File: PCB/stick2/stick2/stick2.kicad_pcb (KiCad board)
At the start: 2 copper layers, 80 x 65.5 mm, 13 parts, among them J1 Conn_01x08_Pin, U1 MLX90395xLW

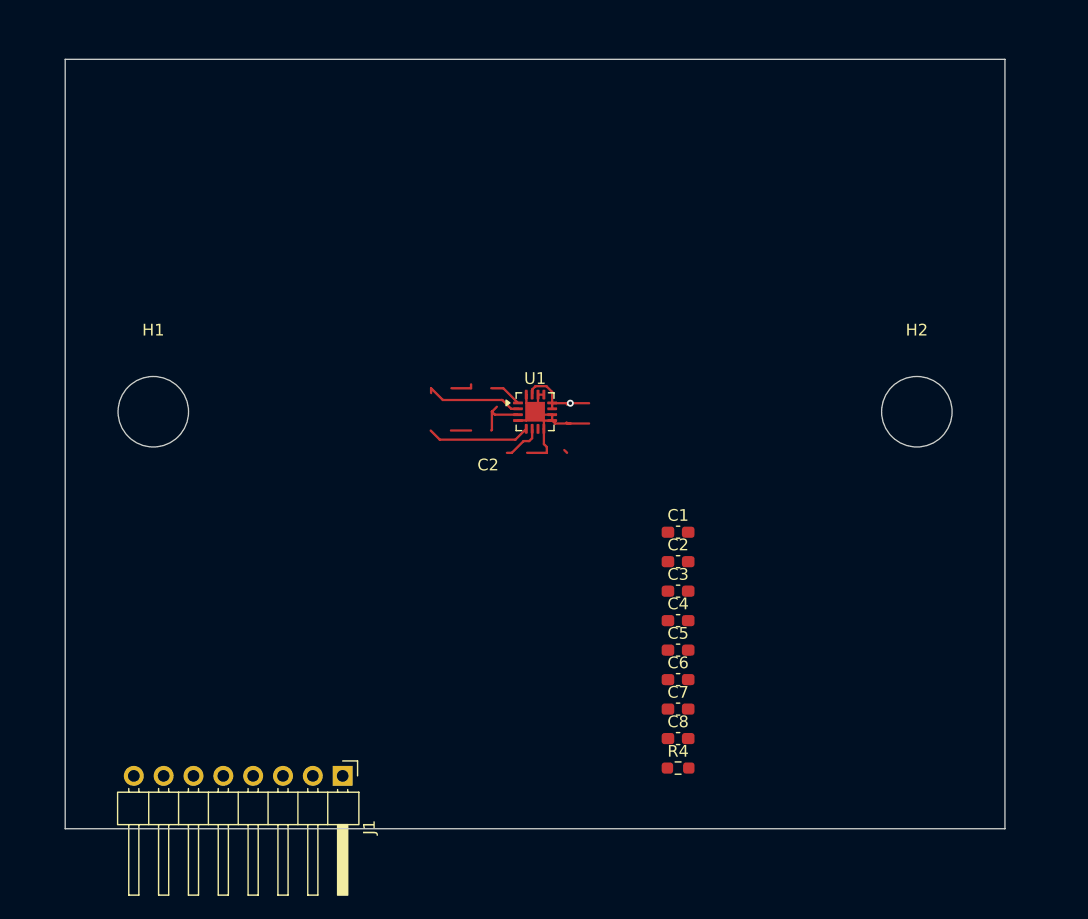
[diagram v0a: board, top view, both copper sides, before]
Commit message: boards
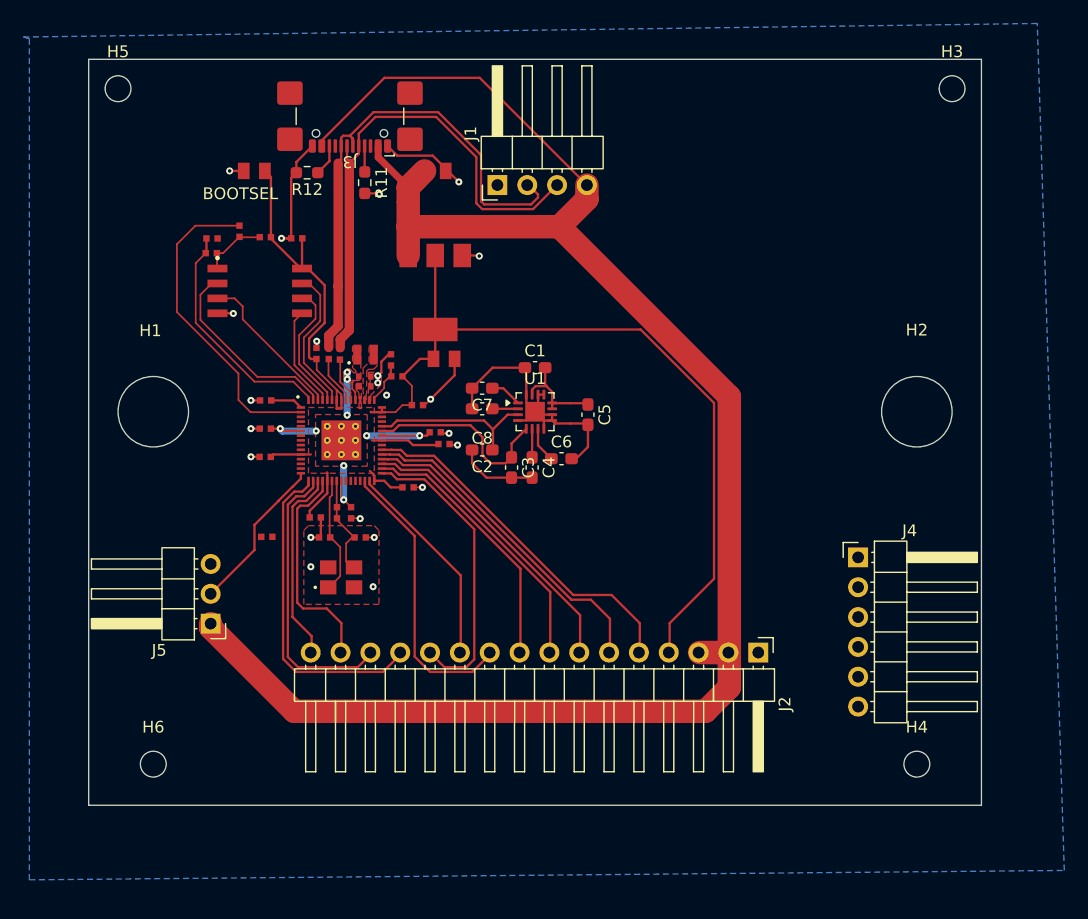
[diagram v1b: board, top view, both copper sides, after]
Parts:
- removed R4: 100, Resistor_SMD:R_0603_1608Metric_Pad0.98x0.95mm_HandSolder
- added C10: 100n, RPI_COMPILED:generic_capc1005x50, F.Cu at (117.1, 79.0)
- added C11: 10u, RPI_COMPILED:generic_capc2012x125, F.Cu at (132.2, 75.5)
- added C12: 15p, RPI_COMPILED:generic_capc1005x50, F.Cu at (122.1, 90.7)
- added C13: 15p, RPI_COMPILED:generic_capc1005x50, F.Cu at (125.1, 90.7)
- added C14: 100n, RPI_COMPILED:generic_capc1005x50, F.Cu at (124.3, 88.6)
- added C15: 100n, RPI_COMPILED:generic_capc1005x50, F.Cu at (131.5, 81.8)
- added C16: 100n, RPI_COMPILED:generic_capc1005x50, F.Cu at (117.0, 81.4)
- added C17: 4.7u, RPI_COMPILED:generic_capc1005x50_wide, F.Cu at (125.5, 77.0)
- added C18: 4.7u, RPI_COMPILED:generic_capc1005x50_wide, F.Cu at (125.5, 77.8)
- added C19: 4.7u, RPI_COMPILED:generic_capc1005x50, F.Cu at (127.7, 75.6)
- added C20: 100n, RPI_COMPILED:generic_capc1005x50, F.Cu at (121.4, 75.0)
- added C21: 100n, RPI_COMPILED:generic_capc1005x50, F.Cu at (130.0, 79.4)
- added C22: 10u, RPI_COMPILED:generic_capc2012x125, F.Cu at (116.1, 59.5)
- added C23: 100n, RPI_COMPILED:generic_capc1005x50, F.Cu at (129.2, 86.4)
- added C24: 100n, RPI_COMPILED:generic_capc1005x50, F.Cu at (121.3, 89.0)
- added C25: 100n, RPI_COMPILED:generic_capc1005x50, F.Cu at (132.2, 82.8)
- added C26: 100n, RPI_COMPILED:generic_capc1005x50, F.Cu at (119.7, 65.2)
- added C27: 100n, RPI_COMPILED:generic_capc1005x50, F.Cu at (117.0, 83.8)
- added C9: 10u, RPI_COMPILED:generic_capc2012x125, F.Cu at (131.5, 59.5)
- added H3: MountingHole, MountingHole:MountingHole_2.2mm_M2, F.Cu at (175.5, 52.5)
- added H4: MountingHole, MountingHole:MountingHole_2.2mm_M2, F.Cu at (172.5, 110.0)
- added H5: MountingHole, MountingHole:MountingHole_2.2mm_M2, F.Cu at (104.5, 52.5)
- added H6: MountingHole, MountingHole:MountingHole_2.2mm_M2, F.Cu at (107.5, 110.0)
- added J2: Conn_01x16, Connector_PinHeader_2.54mm:PinHeader_1x16_P2.54mm_Horizontal, F.Cu at (159.0, 100.5)
- added J3: USB_C_Receptacle_USB2.0_16P, Connector_USB:USB_C_Receptacle_GCT_USB4110, F.Cu at (124.2, 53.7)
- added J4: Conn_01x06_Pin, Connector_PinHeader_2.54mm:PinHeader_1x06_P2.54mm_Horizontal, F.Cu at (167.5, 92.4)
- added J5: Conn_01x03_Pin, Connector_PinHeader_2.54mm:PinHeader_1x03_P2.54mm_Horizontal, F.Cu at (112.4, 98.0)
- added L1: 3.3u, RPI_COMPILED:abracon_aota-b201610s3r3-101-t, F.Cu at (125.6, 75.1)
- added R1: 10k, RPI_COMPILED:generic_resc1005x35, F.Cu at (117.0, 65.1)
- added R10: 0, RPI_COMPILED:generic_resc1005x35, F.Cu at (112.4, 66.5)
- added R11: 5.1k, Resistor_SMD:R_0603_1608Metric_Pad0.98x0.95mm_HandSolder, F.Cu at (125.5, 60.5)
- added R12: 5.1k, Resistor_SMD:R_0603_1608Metric_Pad0.98x0.95mm_HandSolder, F.Cu at (120.6, 59.7)
- added R2: 1k, RPI_COMPILED:generic_resc1005x35, F.Cu at (123.1, 88.6)
- added R3: 33, RPI_COMPILED:generic_resc1005x35, F.Cu at (128.2, 77.0)
- added R5: 1k, RPI_COMPILED:generic_resc1005x35, F.Cu at (117.2, 90.7)
- added R6: 1k, RPI_COMPILED:generic_resc1005x35, F.Cu at (112.5, 65.2)
- added R7: 27, RPI_COMPILED:generic_resc1005x35, F.Cu at (122.4, 75.0)
- added R8: 27, RPI_COMPILED:generic_resc1005x35, F.Cu at (123.4, 75.1)
- added R9: 0, RPI_COMPILED:generic_resc1005x35, F.Cu at (114.8, 64.6)
- added U2: NCP1117ST33T3G, RPI_COMPILED:onsemi_ncp1117st33t3g, F.Cu at (131.5, 69.8)
- added U3: W25Q128JVSIQ, RPI_COMPILED:generic_soic127p790x195-8, F.Cu at (116.6, 69.7)
- added U4: RP2350A, RPI_COMPILED:rpi_rp2350a_vias, F.Cu at (123.5, 82.4)
- added X1: 12MHz, RPI_COMPILED:generic_xtalcc320x250x80-4, F.Cu at (123.5, 94.1)
- J1: value Conn_01x08_Pin -> Conn_01x04_Pin; footprint Connector_PinHeader_2.54mm:PinHeader_1x08_P2.54mm_Horizontal -> Connector_PinHeader_2.54mm:PinHeader_1x04_P2.54mm_Horizontal
- moved J1 52.0 mm to (136.8, 60.7), turned to 90 degrees
- moved C8 32.7 mm to (135.5, 79.8), turned to 180 degrees
- moved C7 32.0 mm to (135.5, 78.0), turned to 180 degrees
- moved C5 21.5 mm to (144.5, 80.2), turned to -90 degrees
- moved C6 21.3 mm to (142.2, 84.0)
- moved C2 19.2 mm to (135.5, 83.2), turned to 180 degrees
- moved C1 18.6 mm to (140.0, 76.2)
- moved C4 18.0 mm to (139.8, 84.8), turned to -90 degrees
- moved C3 17.7 mm to (138.0, 84.8), turned to -90 degrees
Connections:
- net /CS renamed Net-(U1-~{CS})
- net /MISO renamed Net-(U1-MISO)
- net /MOSI renamed /GPIO26_ADC0
- net Net-(U1-SCLK) renamed /GPIO27_ADC1
- J1 pad 1: unconnected-(J1-Pin_1-Pad1) -> GND
- J1 pad 2: unconnected-(J1-Pin_2-Pad2) -> /USB_D+
- J1 pad 3: unconnected-(J1-Pin_3-Pad3) -> /USB_D-
- J1 pad 4: unconnected-(J1-Pin_4-Pad4) -> VBUS
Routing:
- net VBUS: track 0.00 -> 159.0 mm
- net +3V3: track 0.00 -> 117.4 mm
- net /USB_D+: track 0.00 -> 44.7 mm
- net /USB_D-: track 0.00 -> 44.3 mm
- net GND: track 0.00 -> 38.4 mm, vias 0 -> 22
- net /GPIO24: track 0.00 -> 30.7 mm
- net /GPIO23: track 0.00 -> 28.2 mm
- net /GPIO12: track 0.00 -> 27.6 mm
- net /GPIO0: track 0.00 -> 27.1 mm
- net /GPIO22: track 0.00 -> 25.7 mm
- net /GPIO19: track 0.00 -> 25.3 mm
- net +1V1: track 0.00 -> 25.3 mm, vias 0 -> 9
- net /GPIO17: track 0.00 -> 24.4 mm
- net /GPIO13: track 0.00 -> 24.2 mm
- net /GPIO21: track 0.00 -> 24.1 mm
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- added copper zone on F.Cu, net +1V1
- added copper zone on F.Cu, net +3V3
- added copper zone on F.Cu, net /VREG_LX
- added copper zone on B.Cu, net GND
- added copper zone on F.Cu, net GND
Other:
- board size 80 x 65.5 mm -> 76 x 63.5 mm
- board text added: "BOOTSEL"
- board text removed: "C2"
